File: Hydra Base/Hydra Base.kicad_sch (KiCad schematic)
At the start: 2 parts, among them J1 Conn_01x04, U1 Hydra_Core

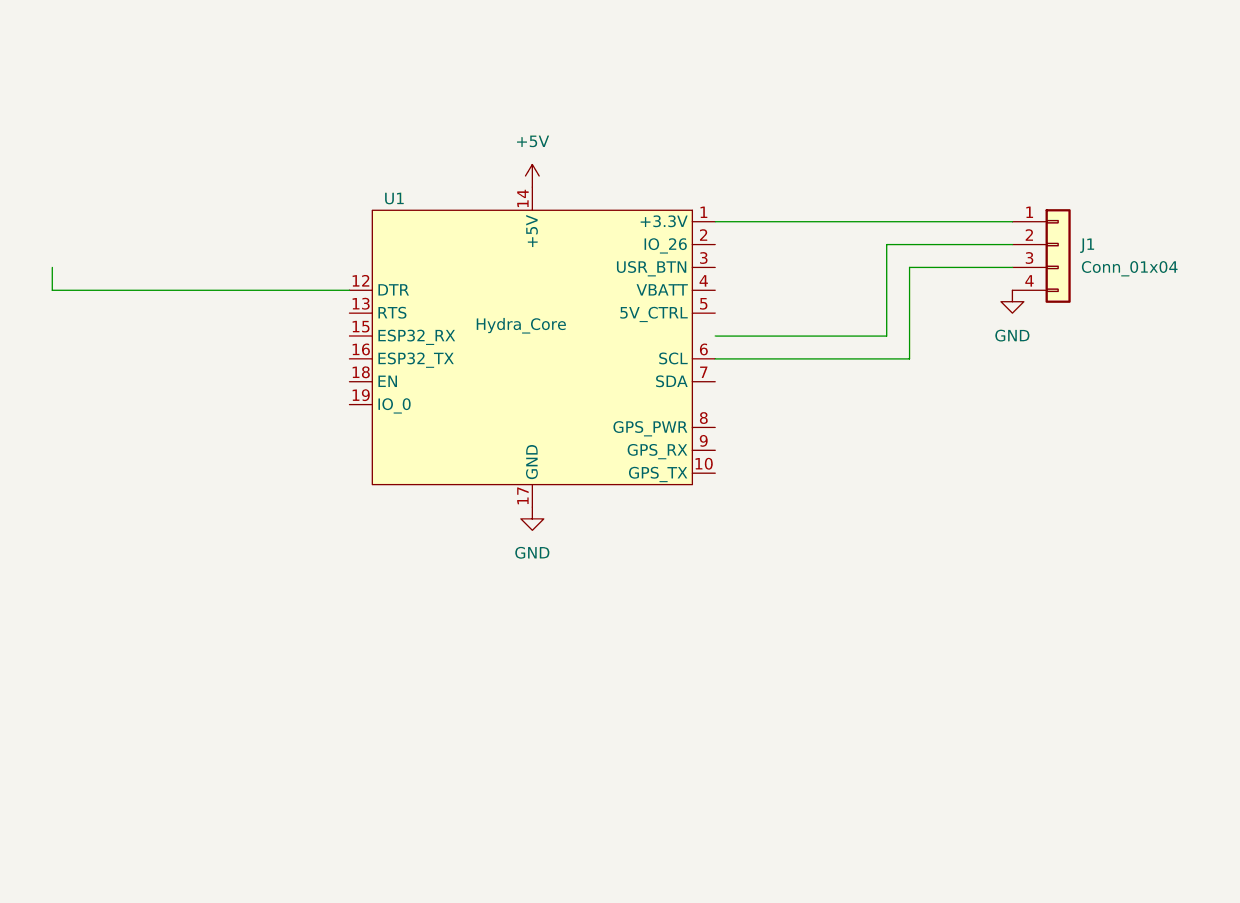
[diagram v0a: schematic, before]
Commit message: Primitive base board example
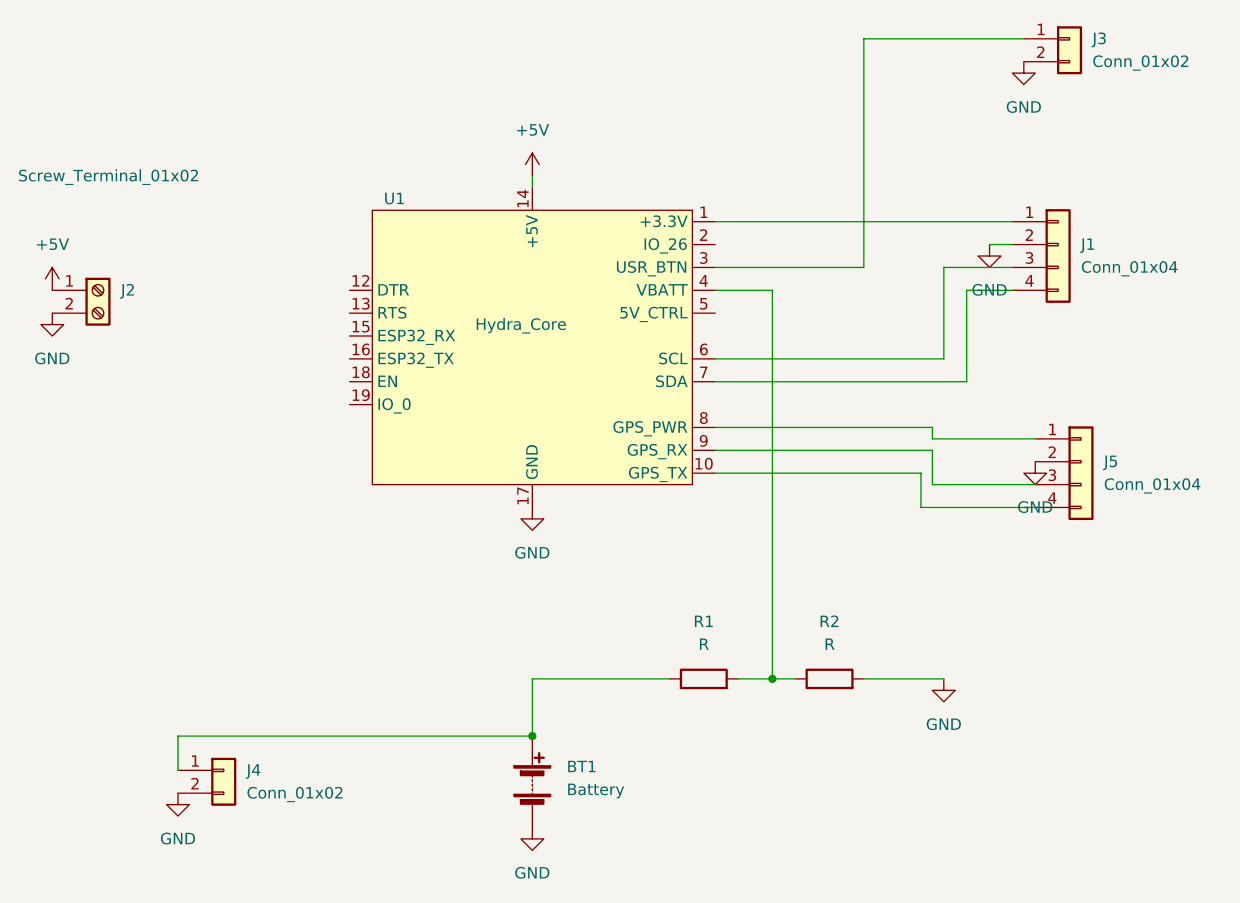
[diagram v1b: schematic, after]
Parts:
- added BT1: Battery, Battery:BatteryHolder_MPD_BH-18650-PC2, symbol Device:Battery
- added J2: Screw_Terminal_01x02, TerminalBlock:TerminalBlock_Altech_AK300-2_P5.00mm, symbol Connector:Screw_Terminal_01x02
- added J3: Conn_01x02, Connector_PinHeader_2.54mm:PinHeader_1x02_P2.54mm_Vertical, symbol Connector_Generic:Conn_01x02
- added J4: Conn_01x02, Connector_JST:JST_PH_B2B-PH-K_1x02_P2.00mm_Vertical, symbol Connector_Generic:Conn_01x02
- added J5: Conn_01x04, Connector_PinHeader_2.54mm:PinHeader_1x04_P2.54mm_Vertical, symbol Connector_Generic:Conn_01x04
- added R1, R2: R, Resistor_THT:R_Axial_DIN0204_L3.6mm_D1.6mm_P5.08mm_Horizontal, symbol Device:R
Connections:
- net +5V: now also J2.1 (Pin_1)
- net GND: now also J1.2 (Pin_2), BT1.2 (-), J2.2 (Pin_2), J3.2 (Pin_2), J4.2 (Pin_2), J5.2 (Pin_2), R2.2; no longer J1.4 (Pin_4)
- net at U1.10 (GPS_TX): now also J5.4 (Pin_4)
- net at U1.3 (USR_BTN): now also J3.1 (Pin_1)
- net at U1.4 (VBATT): now also R1.2, R2.1
- net at U1.7 (SDA): now also J1.4 (Pin_4)
- net at U1.8 (GPS_PWR): now also J5.1 (Pin_1)
- net at U1.9 (GPS_RX): now also J5.3 (Pin_3)
- new net: BT1.1 (+), J4.1 (Pin_1), R1.1
